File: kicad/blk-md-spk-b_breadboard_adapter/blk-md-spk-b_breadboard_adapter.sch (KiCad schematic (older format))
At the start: 4 parts, among them J1 SCJ368R1NUS0B00G, P1 CONNECTOR, P2 CONNECTOR, U1 BLK-MD-SPK-B

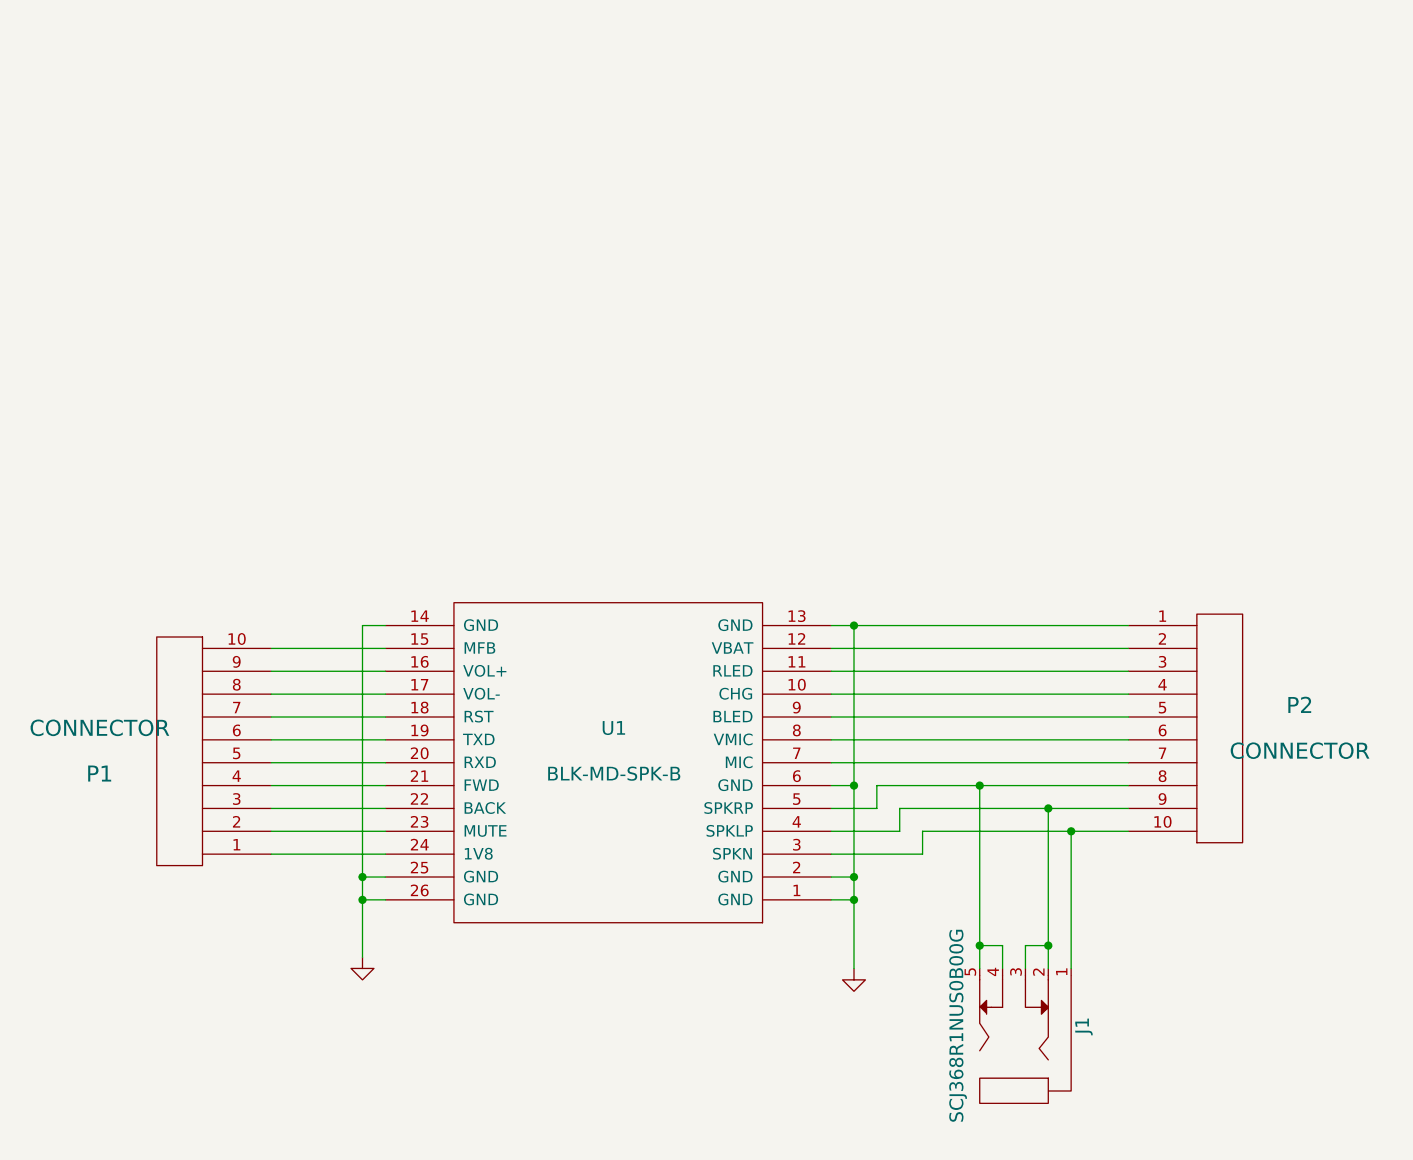
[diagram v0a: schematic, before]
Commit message: updated version
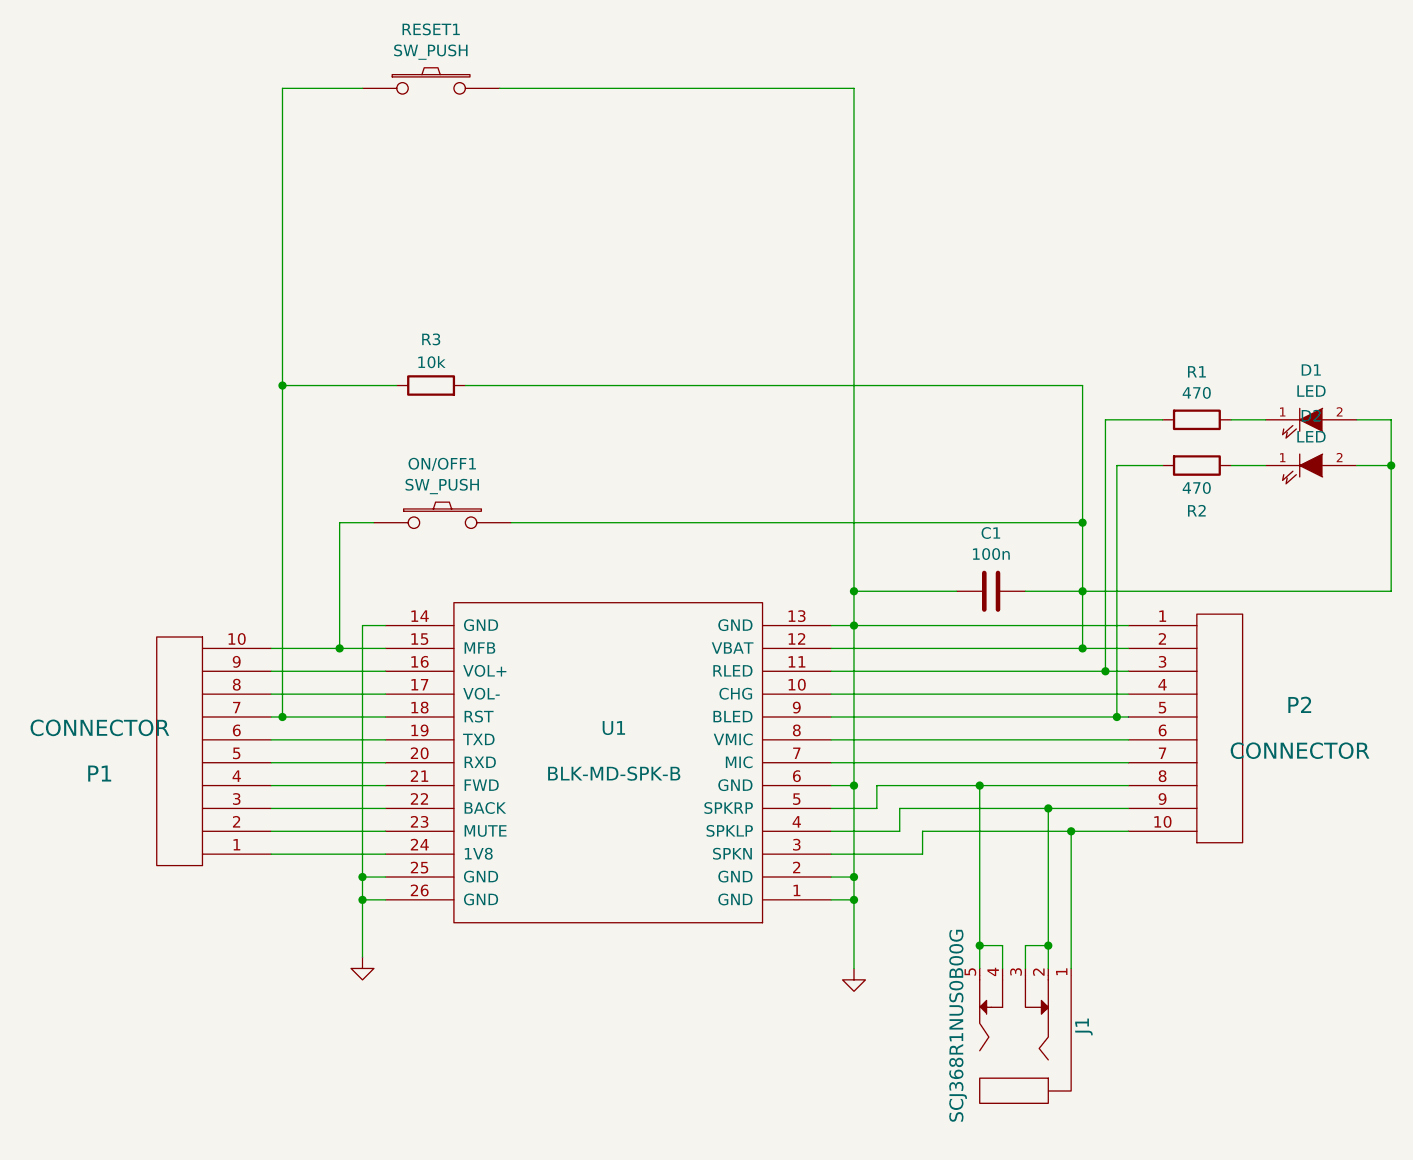
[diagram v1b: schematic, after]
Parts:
- added C1: 100n, Capacitors_SMD:C_0805_HandSoldering, symbol C
- added D1, D2: LED, LEDs:LED-1206, symbol LED
- added ON/OFF1, RESET1: SW_PUSH, Buttons_Switches_SMD:SW_SPST_FSMSM, symbol SW_PUSH
- added R1, R2: 470, Resistors_SMD:R_0805_HandSoldering, symbol R
- added R3: 10k, Resistors_SMD:R_0805_HandSoldering, symbol R
- J1: footprint (none) -> jacks:SCJ-0354-5PU_no_screew
- P1, P2: footprint ~ -> Pin_Headers:Pin_Header_Straight_1x10
- U1: footprint ~ -> my_modules:BLK-MD-SPK-B_no_up_silk
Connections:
- net GND: now also C1.2, RESET1.2
- net at P2.3, U1.11 (RLED): now also R1.2
- net at P2.2, U1.12 (VBAT): now also C1.1, D1.2 (A), D2.2 (A), ON/OFF1.2, R3.2
- net at P1.10, U1.15 (MFB): now also ON/OFF1.1
- net at P1.7, U1.18 (RST): now also R3.1, RESET1.1
- net at P2.5, U1.9 (BLED): now also R2.2
- new net: D1.1 (K), R1.1
- new net: D2.1 (K), R2.1
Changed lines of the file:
@@
 EESchema Schematic File Version 2
-LIBS:bluetooth_breadboard_adapter-rescue
+LIBS:blk-md-spk-b_breadboard_adapter-rescue
 LIBS:power
 LIBS:device
@@
 LIBS:zener
 LIBS:BLK-MD-SPK-B
-LIBS:bluetooth_breadboard_adapter-cache
+LIBS:blk-md-spk-b_breadboard_adapter-cache
 EELAYER 25 0
 EELAYER END
@@
 $EndDescr
 $Comp
-L BLK-MD-SPK-B U1
-U 1 1 54200037
-P 4650 4050
-F 0 "U1" H 4650 3950 60  0000 C CNN
-F 1 "BLK-MD-SPK-B" H 4650 4150 60  0000 C CNN
-F 2 "~" H 4650 4050 60  0000 C CNN
-F 3 "~" H 4650 4050 60  0000 C CNN
-	1    4650 4050
-	-1   0    0    1
-$EndComp
-$Comp
 L CONN_10 P1
 U 1 1 54200046
@@
 F 0 "P1" H 3100 4150 70  0000 C CNN
 F 1 "CONNECTOR" H 3100 3950 70  0000 C CNN
-F 2 "~" H 2750 4050 60  0000 C CNN
+F 2 "Pin_Headers:Pin_Header_Straight_1x10" H 2750 4050 60  0001 C CNN
 F 3 "~" H 2750 4050 60  0000 C CNN
 	1    2750 4050
@@
 F 0 "J1" H 6400 5550 60  0000 C CNN
 F 1 "SCJ368R1NUS0B00G" H 6400 5000 60  0000 C CNN
-F 2 "" H 6400 5250 60  0000 C CNN
+F 2 "jacks:SCJ-0354-5PU_no_screew" H 6400 5250 60  0001 C CNN
 F 3 "" H 6400 5250 60  0000 C CNN
 	1    6400 5250
@@
 F 0 "P2" H 7650 4050 70  0000 C CNN
 F 1 "CONNECTOR" H 7650 3850 70  0000 C CNN
-F 2 "~" H 7300 3950 60  0000 C CNN
+F 2 "Pin_Headers:Pin_Header_Straight_1x10" H 7300 3950 60  0001 C CNN
 F 3 "~" H 7300 3950 60  0000 C CNN
 	1    7300 3950
 	1    0    0    -1
 $EndComp
-Wire Wire Line
-	6350 4900 6350 5000
-Connection ~ 6250 4900
-Wire Wire Line
-	6450 5000 6450 4900
-Wire Wire Line
-	6450 4900 6550 4900
-Connection ~ 6550 4900
-Wire Wire Line
-	6250 4200 6250 5000
-Wire Wire Line
-	5600 3500 6900 3500
-Wire Wire Line
-	5600 4700 5700 4700
-Wire Wire Line
-	5700 3500 5700 5000
-Connection ~ 5700 3500
-Wire Wire Line
-	5600 4600 5700 4600
-Connection ~ 5700 4600
-Wire Wire Line
-	5600 4200 5700 4200
-Connection ~ 5700 4200
-Wire Wire Line
-	5600 4100 6900 4100
-Wire Wire Line
-	5600 4000 6900 4000
-Wire Wire Line
-	5600 3900 6900 3900
-Wire Wire Line
-	5600 3800 6900 3800
-Wire Wire Line
-	5600 3700 6900 3700
-Wire Wire Line
-	5600 3600 6900 3600
-Wire Wire Line
-	6550 4300 6550 5000
-Wire Wire Line
-	6650 4400 6650 5000
-Wire Wire Line
-	3550 3500 3650 3500
-Wire Wire Line
-	3550 4700 3650 4700
-Wire Wire Line
-	3650 4600 3550 4600
-Connection ~ 3550 4600
-Wire Wire Line
-	3150 3600 3650 3600
-Wire Wire Line
-	3650 3700 3150 3700
-Wire Wire Line
-	3150 3800 3650 3800
-Wire Wire Line
-	3150 3900 3650 3900
-Wire Wire Line
-	3650 4000 3150 4000
-Wire Wire Line
-	3150 4100 3650 4100
-Wire Wire Line
-	3650 4200 3150 4200
-Wire Wire Line
-	3150 4300 3650 4300
-Wire Wire Line
-	3650 4400 3150 4400
-Wire Wire Line
-	3150 4500 3650 4500
-Connection ~ 5700 4700
-Wire Wire Line
-	5800 4300 5800 4200
-Wire Wire Line
-	5800 4200 6900 4200
-Wire Wire Line
-	5800 4300 5600 4300
-Wire Wire Line
-	6350 4900 6250 4900
-Connection ~ 6250 4200
-Wire Wire Line
-	5900 4300 6900 4300
-Wire Wire Line
-	5900 4400 5900 4300
-Connection ~ 6550 4300
-Wire Wire Line
-	5600 4400 5900 4400
-Wire Wire Line
-	5600 4500 6000 4500
-Wire Wire Line
-	6000 4500 6000 4400
-Wire Wire Line
-	6000 4400 6900 4400
-Connection ~ 6650 4400
 $Comp
 L GND #PWR01
@@
 	1    0    0    -1
 $EndComp
-Wire Wire Line
-	3550 3500 3550 4950
-$Comp
-L GND #PWR?
+$Comp
+L GND #PWR02
 U 1 1 5652F00B
 P 3550 4950
-F 0 "#PWR?" H 3550 4950 30  0001 C CNN
+F 0 "#PWR02" H 3550 4950 30  0001 C CNN
 F 1 "GND" H 3550 4880 30  0001 C CNN
 F 2 "" H 3550 4950 60  0000 C CNN
@@
 	1    0    0    -1
 $EndComp
+$Comp
+L C C1
+U 1 1 56C2DB63
+P 6300 3350
+F 0 "C1" V 6047 3350 50  0000 C CNN
+F 1 "100n" V 6139 3350 50  0000 C CNN
+F 2 "Capacitors_SMD:C_0805_HandSoldering" V 6139 3350 50  0001 C CNN
+F 3 "" H 6300 3350 50  0000 C CNN
+	1    6300 3350
+	0    1    1    0
+$EndComp
+$Comp
+L R R1
+U 1 1 56C2DCE3
+P 7200 2600
+F 0 "R1" V 6992 2600 50  0000 C CNN
+F 1 "470" V 7084 2600 50  0000 C CNN
+F 2 "Resistors_SMD:R_0805_HandSoldering" V 7084 2600 50  0001 C CNN
+F 3 "" H 7200 2600 50  0000 C CNN
+	1    7200 2600
+	0    1    1    0
+$EndComp
+$Comp
+L R R2
+U 1 1 56C2DD76
+P 7200 2800
+F 0 "R2" V 7400 2800 50  0000 C CNN
+F 1 "470" V 7300 2800 50  0000 C CNN
+F 2 "Resistors_SMD:R_0805_HandSoldering" V 7084 2800 50  0001 R TNN
+F 3 "" H 7200 2800 50  0000 C CNN
+	1    7200 2800
+	0    1    1    0
+$EndComp
+$Comp
+L LED D1
+U 1 1 56C2E4C0
+P 7700 2600
+F 0 "D1" H 7700 2816 50  0000 C CNN
+F 1 "LED" H 7700 2724 50  0000 C CNN
+F 2 "LEDs:LED-1206" H 7700 2600 50  0001 C CNN
+F 3 "" H 7700 2600 50  0000 C CNN
+	1    7700 2600
+	1    0    0    -1
+$EndComp
+$Comp
+L LED D2
+U 1 1 56C2E55A
+P 7700 2800
+F 0 "D2" H 7700 3016 50  0000 C CNN
+F 1 "LED" H 7700 2924 50  0000 C CNN
+F 2 "LEDs:LED-1206" H 7700 2800 50  0001 C CNN
+F 3 "" H 7700 2800 50  0000 C CNN
+	1    7700 2800
+	1    0    0    -1
+$EndComp
+$Comp
+L SW_PUSH RESET1
+U 1 1 56C30A34
+P 3850 1150
+F 0 "RESET1" H 3850 1406 50  0000 C CNN
+F 1 "SW_PUSH" H 3850 1314 50  0000 C CNN
+F 2 "Buttons_Switches_SMD:SW_SPST_FSMSM" H 3850 1314 50  0001 C CNN
+F 3 "" H 3850 1150 50  0000 C CNN
+	1    3850 1150
+	1    0    0    -1
+$EndComp
+$Comp
+L R R3
+U 1 1 56C45ECC
+P 3850 2450
+F 0 "R3" V 4050 2450 50  0000 C CNN
+F 1 "10k" V 3950 2450 50  0000 C CNN
+F 2 "Resistors_SMD:R_0805_HandSoldering" V 3734 2450 50  0001 R TNN
+F 3 "" H 3850 2450 50  0000 C CNN
+	1    3850 2450
+	0    -1   -1   0
+$EndComp
+Wire Wire Line
+	6350 4900 6350 5000
+Connection ~ 6250 4900
+Wire Wire Line
+	6450 5000 6450 4900
+Wire Wire Line
+	6450 4900 6550 4900
+Connection ~ 6550 4900
+Wire Wire Line
+	6250 4200 6250 5000
+Wire Wire Line
+	5600 3500 6900 3500
+Wire Wire Line
+	5600 4700 5700 4700
+Wire Wire Line
+	5700 1150 5700 5000
+Connection ~ 5700 3500
+Wire Wire Line
+	5600 4600 5700 4600
+Connection ~ 5700 4600
+Wire Wire Line
+	5600 4200 5700 4200
+Connection ~ 5700 4200
+Wire Wire Line
+	5600 4100 6900 4100
+Wire Wire Line
+	5600 4000 6900 4000
+Wire Wire Line
+	5600 3900 6900 3900
+Wire Wire Line
+	5600 3800 6900 3800
+Wire Wire Line
+	5600 3700 6900 3700
+Wire Wire Line
+	5600 3600 6900 3600
+Wire Wire Line
+	6550 4300 6550 5000
+Wire Wire Line
+	6650 4400 6650 5000
+Wire Wire Line
+	3550 3500 3650 3500
+Wire Wire Line
+	3550 4700 3650 4700
+Wire Wire Line
+	3650 4600 3550 4600
+Connection ~ 3550 4600
+Wire Wire Line
+	3150 3600 3650 3600
+Wire Wire Line
+	3650 3700 3150 3700
+Wire Wire Line
+	3150 3800 3650 3800
+Wire Wire Line
+	3150 3900 3650 3900
+Wire Wire Line
+	3650 4000 3150 4000
+Wire Wire Line
+	3150 4100 3650 4100
+Wire Wire Line
+	3650 4200 3150 4200
+Wire Wire Line
+	3150 4300 3650 4300
+Wire Wire Line
+	3650 4400 3150 4400
+Wire Wire Line
+	3150 4500 3650 4500
+Connection ~ 5700 4700
+Wire Wire Line
+	5800 4300 5800 4200
+Wire Wire Line
+	5800 4200 6900 4200
+Wire Wire Line
+	5800 4300 5600 4300
+Wire Wire Line
+	6350 4900 6250 4900
+Connection ~ 6250 4200
+Wire Wire Line
+	5900 4300 6900 4300
+Wire Wire Line
+	5900 4400 5900 4300
+Connection ~ 6550 4300
+Wire Wire Line
+	5600 4400 5900 4400
+Wire Wire Line
+	5600 4500 6000 4500
+Wire Wire Line
+	6000 4500 6000 4400
+Wire Wire Line
+	6000 4400 6900 4400
+Connection ~ 6650 4400
+Wire Wire Line
+	3550 3500 3550 4950
 Connection ~ 3550 4700
+Wire Wire Line
+	6150 3350 5700 3350
+Wire Wire Line
+	8050 3350 6450 3350
+Wire Wire Line
+	7900 2600 8050 2600
+Wire Wire Line
+	8050 2600 8050 3350
+Wire Wire Line
+	6700 2450 6700 3600
+Connection ~ 6700 3350
+Connection ~ 6700 3600
+Wire Wire Line
+	7900 2800 8050 2800
+Connection ~ 8050 2800
+Wire Wire Line
+	7500 2600 7350 2600
+Wire Wire Line
+	7350 2800 7500 2800
+Wire Wire Line
+	7050 2800 6850 2800
+Wire Wire Line
+	6850 2800 6850 3900
+Connection ~ 6850 3900
+Wire Wire Line
+	6800 3700 6800 2600
+Wire Wire Line
+	6800 2600 7050 2600
+Connection ~ 6800 3700
+Wire Wire Line
+	3550 1150 3200 1150
+Wire Wire Line
+	3200 1150 3200 3900
+Connection ~ 3200 3900
+Wire Wire Line
+	4150 1150 5700 1150
+Connection ~ 5700 3350
+Wire Wire Line
+	4000 2450 6700 2450
+Wire Wire Line
+	3700 2450 3200 2450
+Connection ~ 3200 2450
+$Comp
+L BLK-MD-SPK-B U1
+U 1 1 54200037
+P 4650 4050
+F 0 "U1" H 4650 3950 60  0000 C CNN
+F 1 "BLK-MD-SPK-B" H 4650 4150 60  0000 C CNN
+F 2 "my_modules:BLK-MD-SPK-B_no_up_silk" H 4650 4050 60  0001 C CNN
+F 3 "~" H 4650 4050 60  0000 C CNN
+	1    4650 4050
+	-1   0    0    1
+$EndComp
+$Comp
+L SW_PUSH ON/OFF1
+U 1 1 56C47C55
+P 3900 3050
+F 0 "ON/OFF1" H 3900 3306 50  0000 C CNN
+F 1 "SW_PUSH" H 3900 3214 50  0000 C CNN
+F 2 "Buttons_Switches_SMD:SW_SPST_FSMSM" H 3900 3214 50  0001 C CNN
+F 3 "" H 3900 3050 50  0000 C CNN
+	1    3900 3050
+	1    0    0    -1
+$EndComp
+Wire Wire Line
+	6700 3050 4200 3050
+Connection ~ 6700 3050
+Wire Wire Line
+	3600 3050 3450 3050
+Wire Wire Line
+	3450 3050 3450 3600
+Connection ~ 3450 3600
 $EndSCHEMATC

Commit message: updates, I do not remember what I changed ....
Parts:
- J1: footprint jacks:SCJ-0354-5PU_no_screew -> jacks:3.5mm_stereo_jack_PJ320B
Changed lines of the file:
@@
 LIBS:zener
 LIBS:BLK-MD-SPK-B
+LIBS:68HC05
+LIBS:aimtec
+LIBS:F-3188_CSR8645
+LIBS:MB-CM15113
+LIBS:raspberryPi_HAT
+LIBS:S3860M-S
+LIBS:SOYO-BT24G03
 LIBS:blk-md-spk-b_breadboard_adapter-cache
 EELAYER 25 0
@@
 F 0 "J1" H 6400 5550 60  0000 C CNN
 F 1 "SCJ368R1NUS0B00G" H 6400 5000 60  0000 C CNN
-F 2 "jacks:SCJ-0354-5PU_no_screew" H 6400 5250 60  0001 C CNN
+F 2 "jacks:3.5mm_stereo_jack_PJ320B" H 6400 5250 60  0001 C CNN
 F 3 "" H 6400 5250 60  0000 C CNN
 	1    6400 5250
